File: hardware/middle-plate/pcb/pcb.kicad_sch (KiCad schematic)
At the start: 113 parts, among them SW1 MT-0-102-A101-M200-RS+PJ, SW2 TS4535TP 250GF 009, SW3 TS4535TP 250GF 009, SW4 TS4535TP 250GF 009, SW5 TS4535TP 250GF 009, SW6 TS4535TP 250GF 009, SW7 TS4535TP 250GF 009

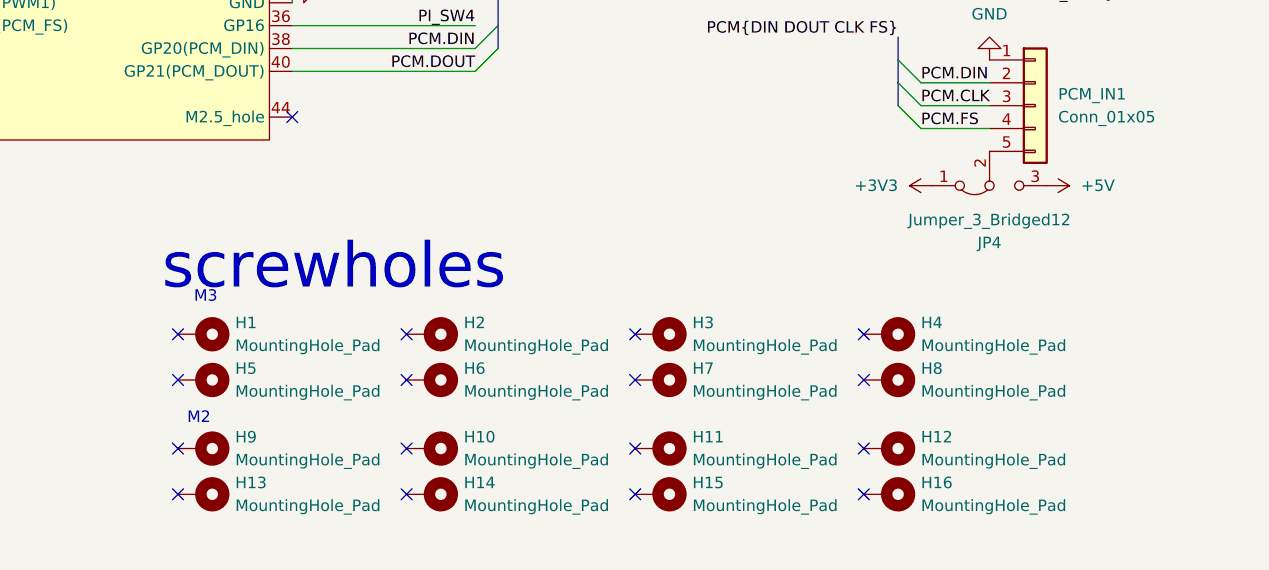
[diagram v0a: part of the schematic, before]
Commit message: fixed middle plate and added stuff to gitignore
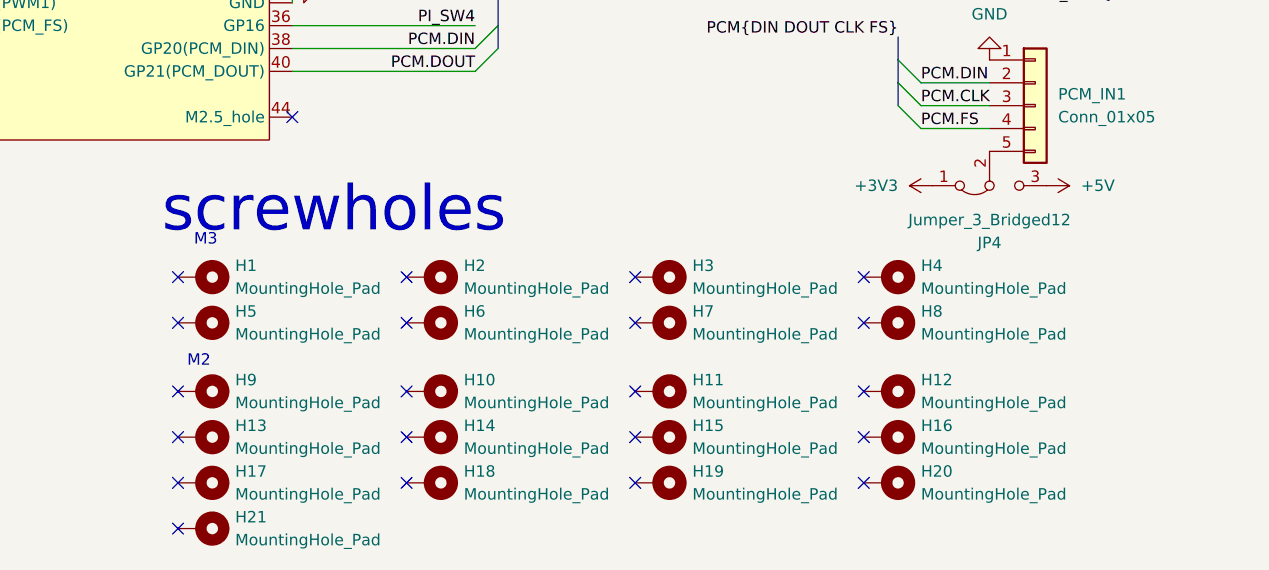
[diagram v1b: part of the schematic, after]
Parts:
- added H17, H18, H19, H20, H21: MountingHole_Pad, MountingHole:MountingHole_2.2mm_M2_Pad_Via, symbol Mechanical:MountingHole_Pad
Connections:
- no-connect marks 28 -> 33
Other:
- moved on the sheet: H1, H10, H11, H12, H13, H14, H15, H16, H2, H3, H4, H5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
